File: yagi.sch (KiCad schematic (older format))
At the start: 59 parts, among them IC1 AT24CS32-SSHM, J1 RPi_GPIO, P1 HV+, P10 CONN_01X02, P11 CONN_01X02, P12 CONN_01X03, P13 CONN_01X01, P14 CONN_01X01, P2 HV-, P3 CONN_01X01, P4 CONN_01X01, P5 CONN_01X02, P6 CONN_01X03, P7 CONN_01X02, P8 CONN_01X03, P9 CONN_01X03, Q1 STN0214, Q2 STN0214, Q3 MMBT4401, U1 74LS244

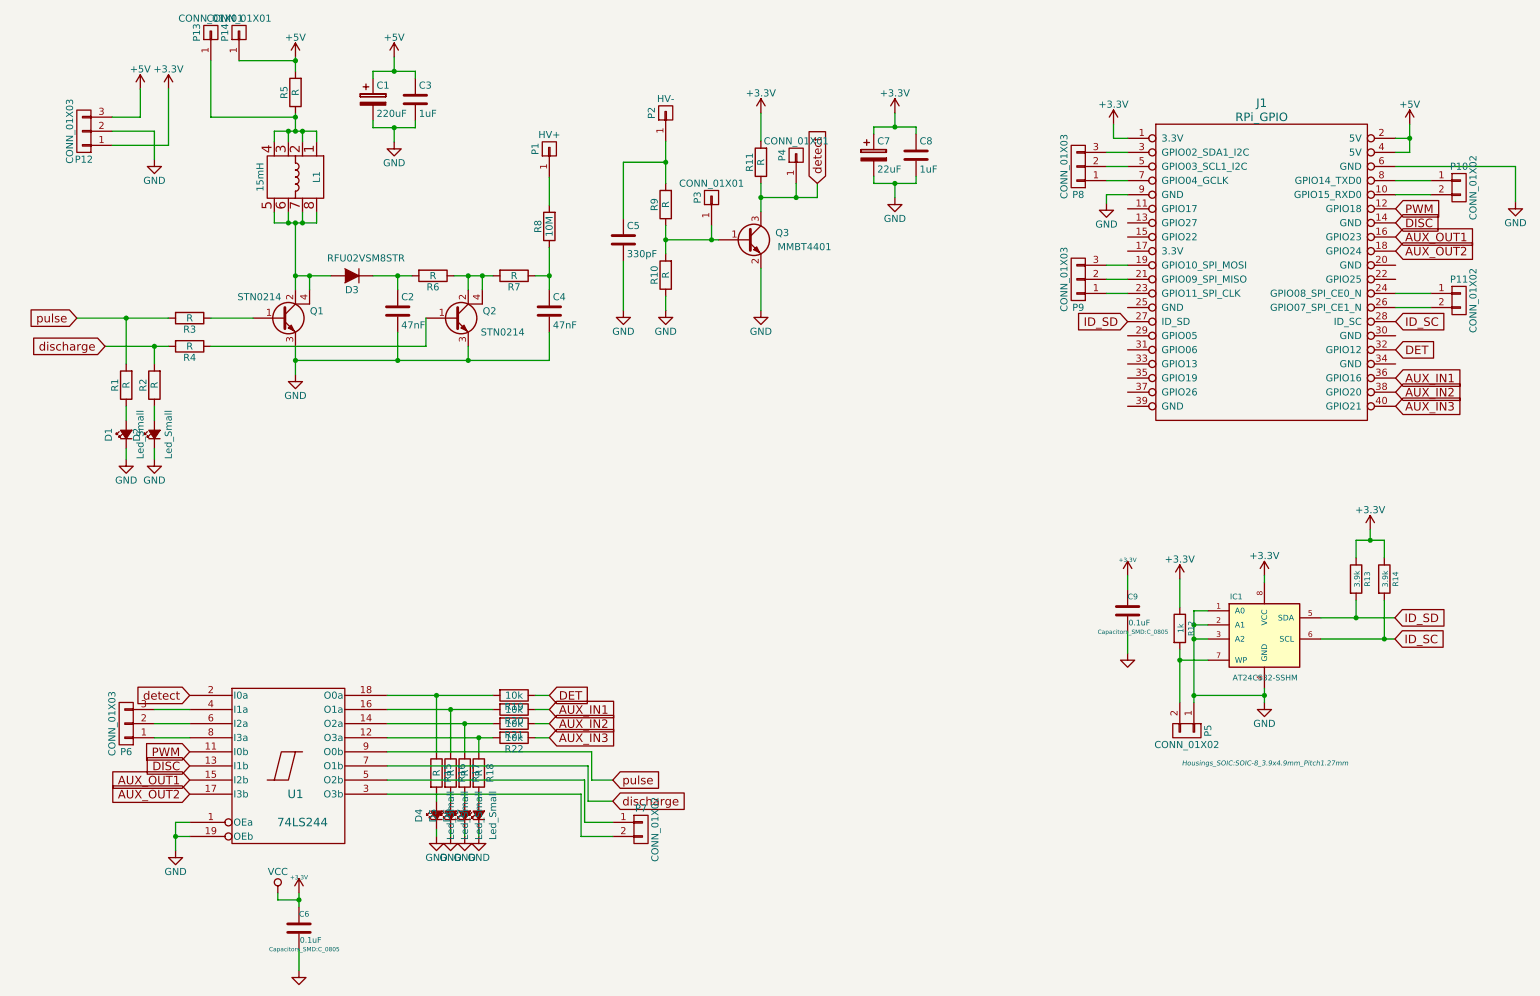
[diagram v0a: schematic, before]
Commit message: New try.
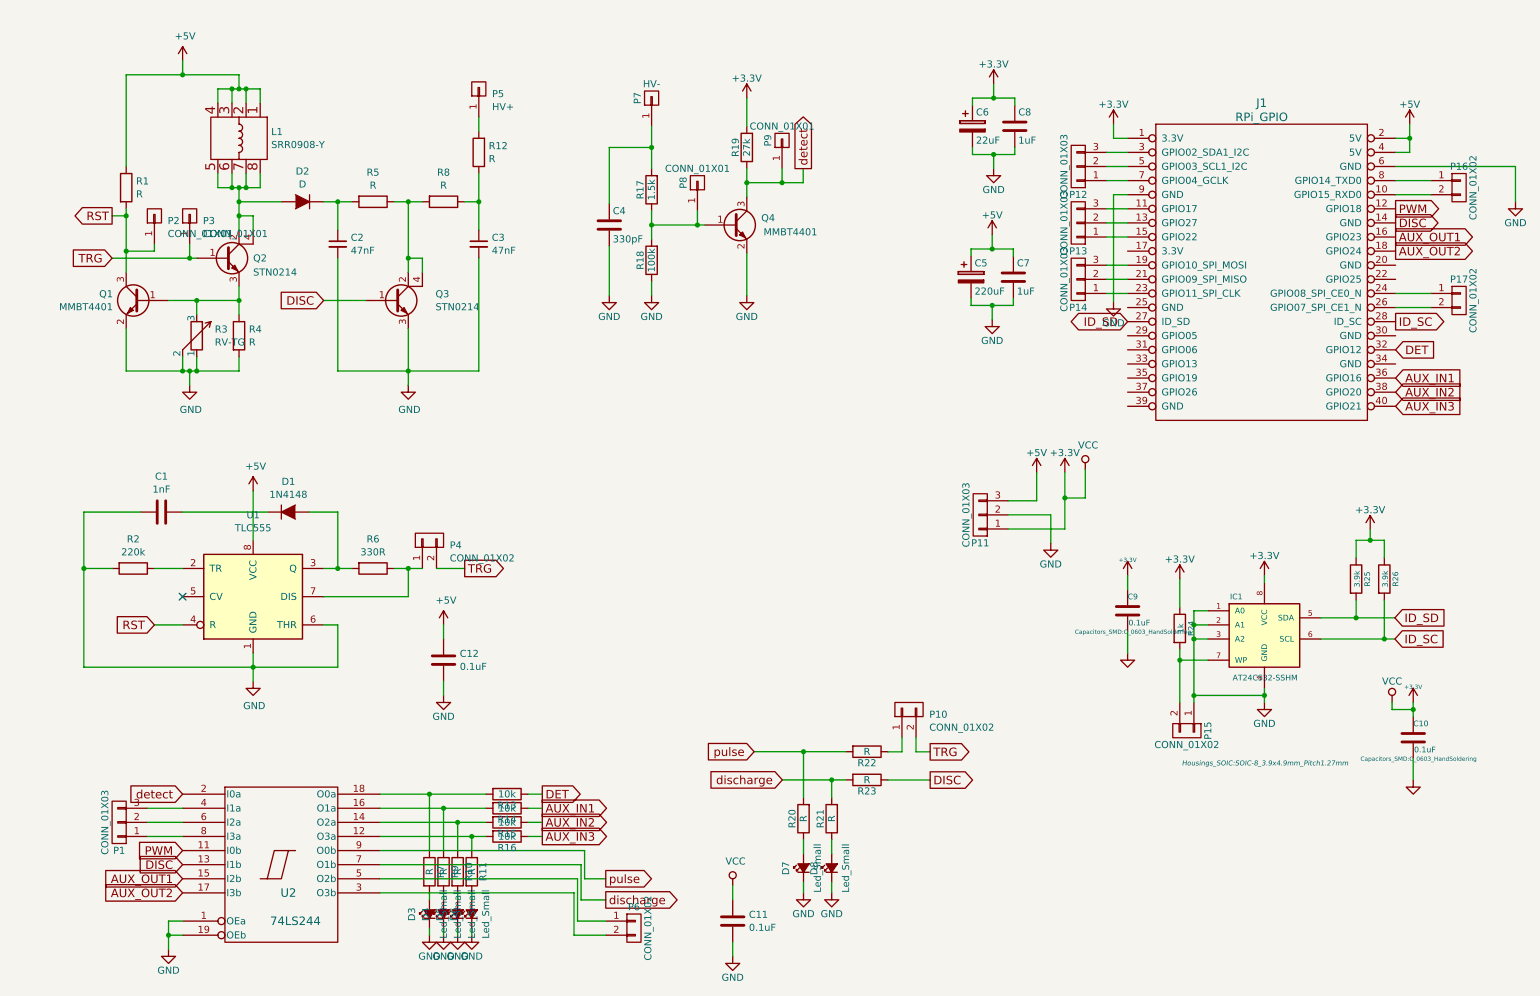
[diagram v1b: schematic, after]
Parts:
- removed C2, C4: 47nF, Capacitors_SMD:C_0805, symbol C
- removed D3: RFU02VSM8STR, chenit:TUMD2SM, symbol D
- removed P1: HV+, Wire_Pads:SolderWirePad_single_1-2mmDrill, symbol CONN_01X01
- removed P13, P14: CONN_01X01, Wire_Pads:SolderWirePad_single_0-8mmDrill, symbol CONN_01X01
- removed Q1: STN0214, chenit:SOT223, symbol Q_NPN_BCEC
- removed R7: R, Resistors_SMD:R_0805_HandSoldering, symbol R
- added C1: 1nF, Capacitors_SMD:C_0805_HandSoldering, symbol C
- added C11, C12: 0.1uF, Capacitors_SMD:C_0603_HandSoldering, symbol C
- added C2, C3: 47nF, Capacitors_SMD:C_1210_HandSoldering, symbol C_Small
- added D1: 1N4148, Discret:DO-35, symbol D
- added D2: D, chenit:TUMD2SM, symbol D
- added P10, P4: CONN_01X02, Pin_Headers:Pin_Header_Straight_1x02, symbol CONN_01X02
- added P13: CONN_01X03, Pin_Headers:Pin_Header_Straight_1x03, symbol CONN_01X03
- added P2, P3: CONN_01X01, chenit:PIN, symbol CONN_01X01
- added P5: HV+, Wire_Pads:SolderWirePad_single_1-2mmDrill, symbol CONN_01X01
- added Q1: MMBT4401, TO_SOT_Packages_SMD:SOT-23, symbol Q_NPN_BEC
- added Q3: STN0214, TO_SOT_Packages_SMD:SOT-223, symbol Q_NPN_BCEC
- added R1, R12, R4: R, Resistors_SMD:R_0805_HandSoldering, symbol R
- added R2: 220k, Resistors_SMD:R_0805_HandSoldering, symbol R
- added R3: RV-TG, chenit:bourns-3361-p, symbol RV-TG
- added U1: TLC555, Housings_SOIC:SOIC-8_3.9x4.9mm_Pitch1.27mm, symbol TLC555
- C10: renamed from C6; footprint Capacitors_SMD:C_0805 -> Capacitors_SMD:C_0603_HandSoldering
- C4: renamed from C5; footprint Capacitors_SMD:C_0603 -> Capacitors_SMD:C_0603_HandSoldering
- C7: renamed from C3; footprint Capacitors_SMD:C_0603 -> Capacitors_SMD:C_0805_HandSoldering
- C8: footprint Capacitors_SMD:C_0805 -> Capacitors_SMD:C_0805_HandSoldering
- C9: footprint Capacitors_SMD:C_0805 -> Capacitors_SMD:C_0603_HandSoldering
- L1: value 15mH -> SRR0908-Y
- Q2: footprint chenit:SOT223 -> TO_SOT_Packages_SMD:SOT-223
- R17: renamed from R9; value R -> 1.5k
- R18: renamed from R10; value R -> 100k
- R19: renamed from R11; value R -> 27k
- R6: value R -> 330R
- R8: value 10M -> R
- U2: renamed from U1; footprint Housings_SOIC:SOIC-20_7.5x12.8mm_Pitch1.27mm -> Housings_SSOP:TSSOP-20_4.4x6.5mm_Pitch0.65mm
- renumbered C1 to C5, C7 to C6, D4 to D3, D5 to D4, D6 to D5, D7 to D6, D1 to D7, D2 to D8, P6 to P1, P12 to P11, P8 to P12, P9 to P14, P5 to P15, P10 to P16, P11 to P17, P7 to P6, P2 to P7, P3 to P8, P4 to P9, Q3 to Q4, R17 to R10, R18 to R11, R19 to R13, R20 to R14, R21 to R15, R22 to R16, R1 to R20, R2 to R21, R3 to R22, R4 to R23, R12 to R24, R13 to R25, R14 to R26, R15 to R7, R16 to R9
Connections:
- net +3V3: now also C11.1
- net +5V: now also L1.1, L1.2, L1.3, L1.4, C12.1, R1.1, U1.8 (VCC); no longer R5.2
- net DISC: now also Q3.1 (B)
- net GND: now also C1.2, C11.2, C12.2, C2.2, C3.2, Q1.2 (E), Q3.3 (E), R2.2, R3.1, R3.2, R4.2, U1.1 (GND), U1.6 (THR); no longer Q2.3 (E)
- net at R6.2: now also D1.2 (A), U1.3 (Q)
- net at L1.5, L1.6, L1.7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: now also Q2.2 (C), Q2.4 (C), D2.2 (A)
- net at R8.1: now also C3.1, R12.1
- net at R8.2: now also R5.1, Q3.2 (C), Q3.4 (C)
- net at R23.1: no longer Q2.1 (B)
- net at J1.11 (GPIO17): now also P13.3 (P3)
- net at J1.13 (GPIO27): now also P13.2 (P2)
- net at J1.15 (GPIO22): now also P13.1 (P1)
- new net: Q1.1 (B), Q2.3 (E), R3.3, R4.1
- new net: C2.1, D2.1 (K), R5.2
- new net: P5.1 (P1), R12.2
- new net: R2.1, U1.2 (TR)
- new net: P4.1 (P1), R6.1, U1.7 (DIS)
- new net: C1.1, D1.1 (K)
- new net RST: P2.1 (P1), Q1.3 (C), R1.2, U1.4 (R)
- new net TRG: P10.2 (P2), P3.1 (P1), P4.2 (P2), Q2.1 (B)
- no-connect marks 0 -> 1
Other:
- moved on the sheet: C10, C4, C5, C6, C7, C8, D3, D4, D5, D6, D7, D8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
